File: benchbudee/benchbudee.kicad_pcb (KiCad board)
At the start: 2 copper layers, 2 parts

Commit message: Setting up for layout
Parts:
- moved Arduino MEGA 392.1 mm to (-186.9, 90.4)
- moved Arduino UNO 392.1 mm to (-186.9, 33.3)
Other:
- board outline added: 165.1 x 63.5 mm
- copper layers 2 -> 4
- rule trace_min: 0.254 -> 0.1524
- rule via_min_drill: 0.508 -> 0.3302
- rule via_min_size: 0.889 -> 0.508
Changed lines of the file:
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@@
-(kicad_pcb (version 3) (host pcbnew "(2013-07-07 BZR 4022)-stable")
+(kicad_pcb (version 3) (host pcbnew "(2014-03-08 BZR 4739)-product")
   (general
     (links 0)
     (no_connects 0)
-    (area 157.150999 89.341 265.759001 204.029)
+    (area 157.150999 88.991 265.759001 204.229)
     (thickness 1.6)
-    (drawings 0)
+    (drawings 4)
     (tracks 0)
     (zones 0)
@@
   (layers
     (15 F.Cu signal)
+    (2 PWR power)
+    (1 GND power)
     (0 B.Cu signal)
     (16 B.Adhes user)
@@
     (22 B.Mask user)
     (23 F.Mask user)
-    (24 Dwgs.User user)
-    (25 Cmts.User user)
-    (26 Eco1.User user)
-    (27 Eco2.User user)
     (28 Edge.Cuts user)
   )
   (setup
     (last_trace_width 0.254)
+    (user_trace_width 0.1524)
     (trace_clearance 0.254)
     (zone_clearance 0.508)
     (zone_45_only no)
-    (trace_min 0.254)
+    (trace_min 0.1524)
     (segment_width 0.2)
     (edge_width 0.1)
     (via_size 0.889)
     (via_drill 0.635)
-    (via_min_size 0.889)
-    (via_min_drill 0.508)
+    (via_min_size 0.508)
+    (via_min_drill 0.3302)
+    (user_via 0.508 0.3302)
     (uvia_size 0.508)
     (uvia_drill 0.127)
     (uvias_allowed no)
-    (uvia_min_size 0.508)
+    (uvia_min_size 0.381)
     (uvia_min_drill 0.127)
     (pcb_text_width 0.3)
@@
   )
   (module Arduino_UNO (layer F.Cu)
-    (at 195.58 119.38)
+    (at -186.944 33.274)
     (fp_text reference "Arduino UNO" (at 0 -29.21) (layer F.SilkS) hide
       (effects (font (size 1 1) (thickness 0.15)))
@@
   )
   (module Arduino_MEGA (layer F.Cu)
-    (at 195.58 176.53)
+    (at -186.944 90.424)
     (fp_text reference "Arduino MEGA" (at 0 -29.21) (layer F.SilkS) hide
       (effects (font (size 1 1) (thickness 0.15)))
@@
     (fp_line (start -31.75 -25.4) (end -31.75 25.4) (layer Eco1.User) (width 0.15))
   )
+  (gr_line (start 110.236 111.76) (end 110.236 175.26) (angle 90) (layer Edge.Cuts) (width 0.1))
+  (gr_line (start 275.336 111.76) (end 110.236 111.76) (angle 90) (layer Edge.Cuts) (width 0.1))
+  (gr_line (start 275.336 175.26) (end 275.336 111.76) (angle 90) (layer Edge.Cuts) (width 0.1))
+  (gr_line (start 110.236 175.26) (end 275.336 175.26) (angle 90) (layer Edge.Cuts) (width 0.1))
 )

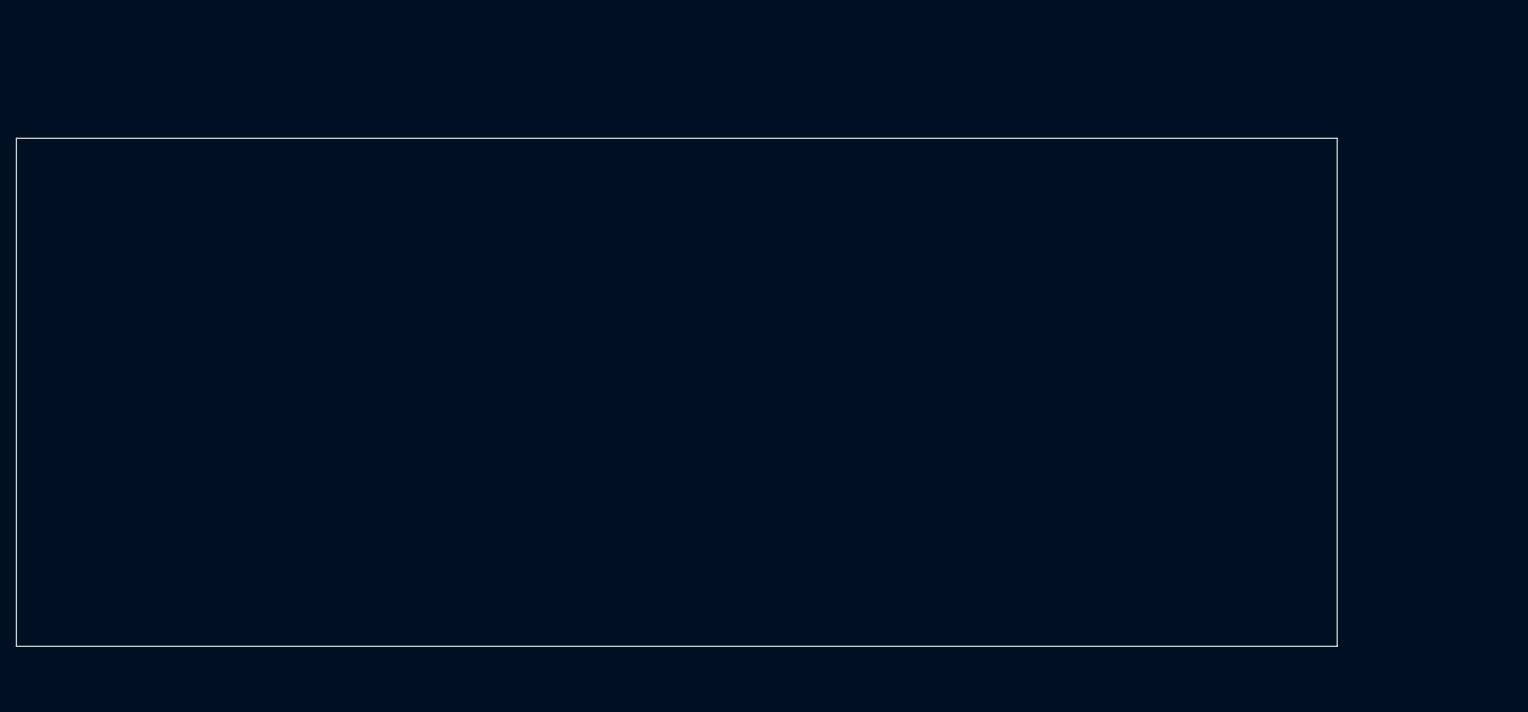
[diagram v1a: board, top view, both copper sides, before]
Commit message: Relay module footprints done
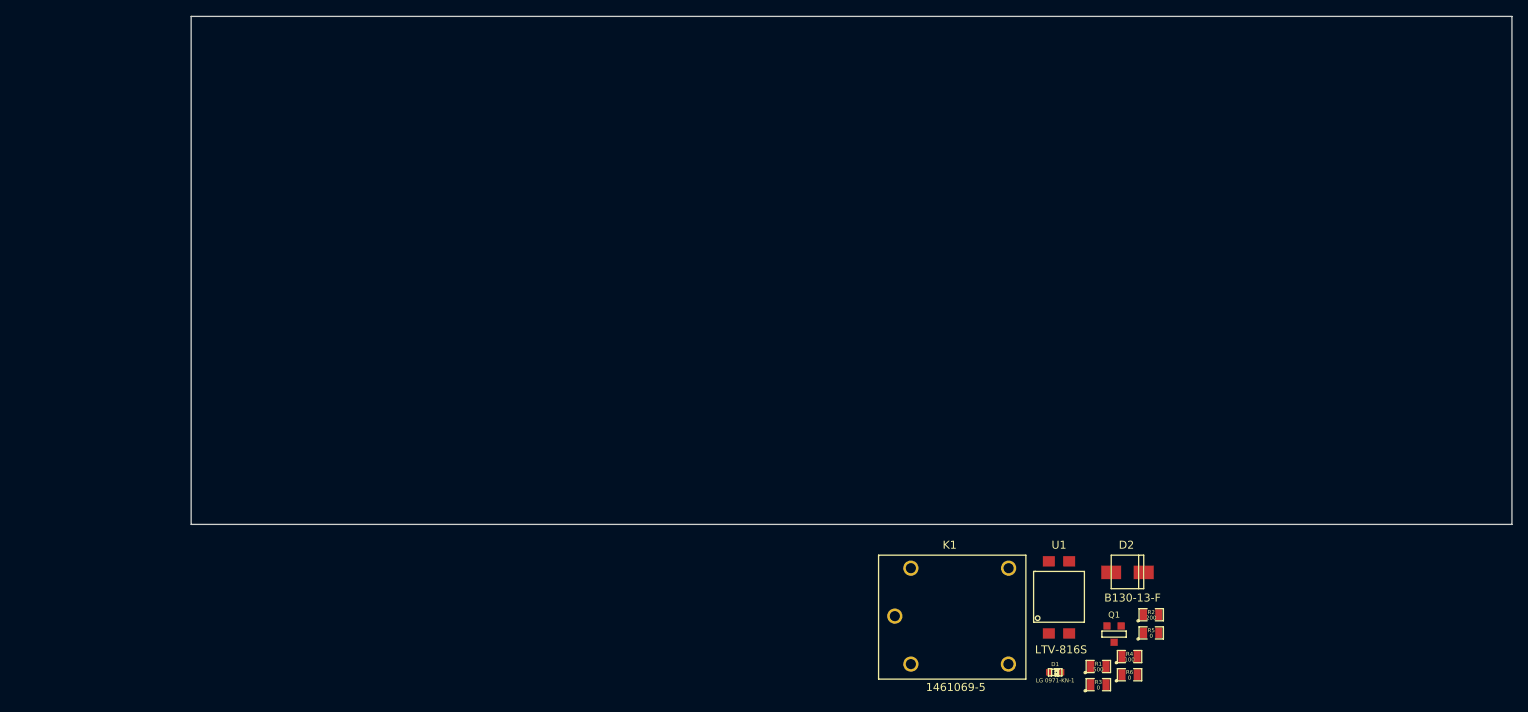
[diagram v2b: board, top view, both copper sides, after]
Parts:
- removed Arduino MEGA: Val**, Arduino_MEGA
- removed Arduino UNO: Val**, Arduino_UNO
- added D1: LG 0971-KN-1, LEDs:LED-0603, F.Cu at (240.1, 178.5)
- added D2: B130-13-F, BenchBudEE:SMA, F.Cu at (247.1, 166.0)
- added K1: 1461069-5, BenchBudEE:TE-SPDT, F.Cu at (220.0, 171.5)
- added Q1: 2N3904, SMD_Packages:SOT23EBC, F.Cu at (247.4, 173.7)
- added R1: 500, SMD_Packages:SM0805, F.Cu at (245.5, 177.8)
- added R2: 200, SMD_Packages:SM0805, F.Cu at (252.1, 171.3)
- added R3: 0, SMD_Packages:SM0805, F.Cu at (245.5, 180.1)
- added R4: 100, SMD_Packages:SM0805, F.Cu at (249.4, 176.5)
- added R5: 0, SMD_Packages:SM0805, F.Cu at (252.1, 173.6)
- added R6: 0, SMD_Packages:SM0805, F.Cu at (249.4, 178.8)
- added U1: LTV-816S, BenchBudEE:4-SMD, F.Cu at (239.3, 173.6)
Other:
- rule pad_to_mask_clearance: 0 -> 0.254
